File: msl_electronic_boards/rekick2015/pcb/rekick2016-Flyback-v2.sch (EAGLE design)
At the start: 201 parts, among them IC1 74LVC1G02GW, IC2 4043D, IC3 LM1117, IC4 LM1458D, P1 39-30-06_S, P2 39-30-08_S, Q1 16MHz, Q2 IKW 25N120, Q3 PSMN7R8-120PS, Q5 IPD90P04P4L, Q6 IRF840, T1 BC859, T2 BC849, T3 BC849, T4 BC849, T5 IRLML6344TRPBF, T6 BC859, U1 TXB0108PWR, U3 LM2675, U4 LM2675, U5 ADUM4190BRIZ, U6 ADUM4190BRIZ, X1 79109-12, X2 79109-04

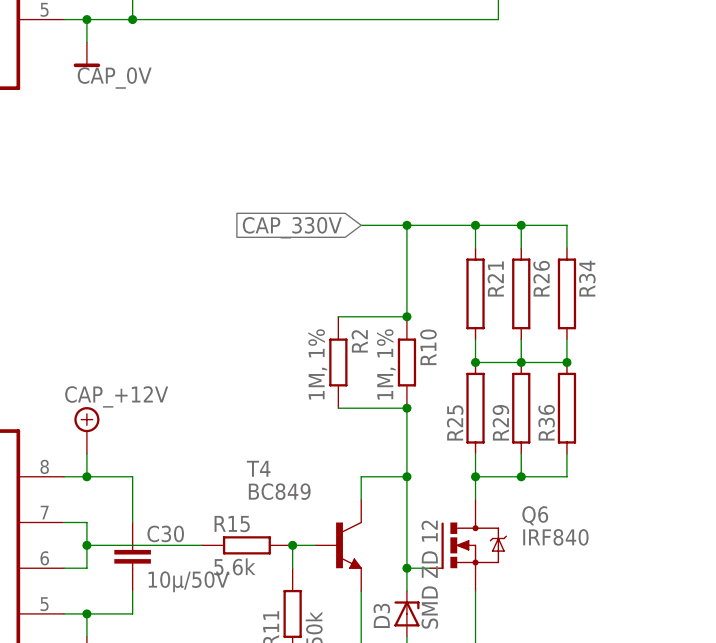
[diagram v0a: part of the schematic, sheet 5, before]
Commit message: rekick board  and  powerswitch board changes
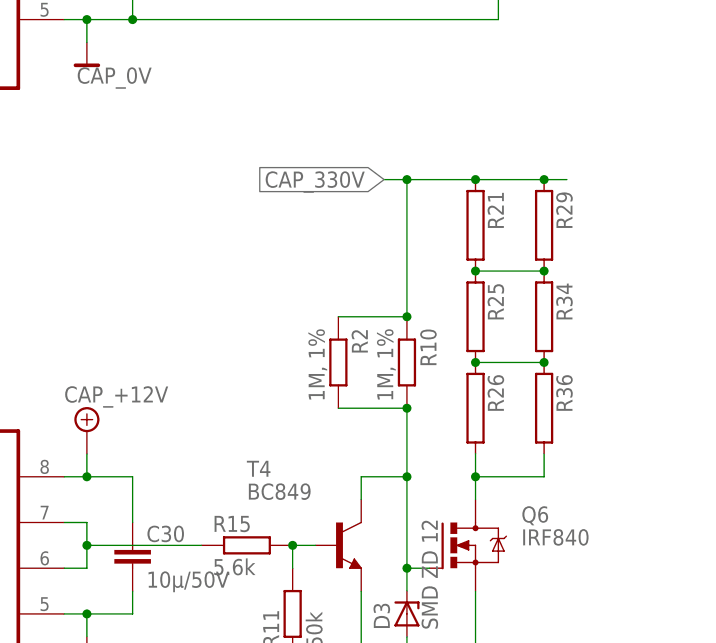
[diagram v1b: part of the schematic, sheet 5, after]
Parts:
- R21, R25, R26, R29, R34, R36: device resistor-power:RKH208-8R -> resistor-power:RKH214-8R
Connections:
- new net N$8: R25.2, R26.1, R34.2, R36.1
- net CAP_330V: now also R29.1; no longer R26.1, R34.1
- net N$13: now also R25.1, R34.1; no longer R25.2, R26.2, R34.2, R36.2
- net N$51: now also R26.2, R36.2; no longer R25.1, R29.1, R36.1
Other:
- moved on the sheet: R21, R25, R26, R29, R34, R36
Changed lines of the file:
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@@
 <part name="SUPPLY20" library="supply2" deviceset="0V" device="" value="CAP_0V"/>
 <part name="GND29" library="supply1" deviceset="GND" device=""/>
-<part name="R21" library="resistor-power" deviceset="R" device="KH208-8R"/>
-<part name="R25" library="resistor-power" deviceset="R" device="KH208-8R"/>
-<part name="R26" library="resistor-power" deviceset="R" device="KH208-8R"/>
-<part name="R29" library="resistor-power" deviceset="R" device="KH208-8R"/>
+<part name="R21" library="resistor-power" deviceset="R" device="KH214-8R"/>
+<part name="R25" library="resistor-power" deviceset="R" device="KH214-8R"/>
+<part name="R26" library="resistor-power" deviceset="R" device="KH214-8R"/>
+<part name="R29" library="resistor-power" deviceset="R" device="KH214-8R"/>
 <part name="FRAME8" library="frames" deviceset="A4L-LOC" device=""/>
 <part name="GND30" library="supply1" deviceset="GND" device=""/>
@@
 <part name="SUPPLY23" library="supply2" deviceset="GND1" device=""/>
 <part name="GND41" library="supply1" deviceset="GND" device=""/>
-<part name="R34" library="resistor-power" deviceset="R" device="KH208-8R"/>
-<part name="R36" library="resistor-power" deviceset="R" device="KH208-8R"/>
+<part name="R34" library="resistor-power" deviceset="R" device="KH214-8R"/>
+<part name="R36" library="resistor-power" deviceset="R" device="KH214-8R"/>
 <part name="X1" library="con-molex-milli-grid" deviceset="79109-12" device=""/>
 <part name="C43" library="rcl" deviceset="C-EU" device="C1206" value="10µ/50V"/>
@@
 <instance part="R11" gate="G$1" x="119.38" y="66.04" rot="R90"/>
 <instance part="R2" gate="G$1" x="124.46" y="93.98" rot="R270"/>
-<instance part="R21" gate="G$1" x="139.7" y="101.6" rot="R270"/>
-<instance part="R25" gate="G$1" x="139.7" y="88.9" rot="R90"/>
-<instance part="R26" gate="G$1" x="144.78" y="101.6" rot="R270"/>
-<instance part="R29" gate="G$1" x="144.78" y="88.9" rot="R90"/>
-<instance part="R34" gate="G$1" x="149.86" y="101.6" rot="R270"/>
-<instance part="R36" gate="G$1" x="149.86" y="88.9" rot="R90"/>
+<instance part="R21" gate="G$1" x="139.7" y="109.22" rot="R270"/>
+<instance part="R25" gate="G$1" x="139.7" y="99.06" rot="R270"/>
+<instance part="R26" gate="G$1" x="139.7" y="88.9" rot="R270"/>
+<instance part="R29" gate="G$1" x="147.32" y="109.22" rot="R270"/>
+<instance part="R34" gate="G$1" x="147.32" y="99.06" rot="R270"/>
+<instance part="R36" gate="G$1" x="147.32" y="88.9" rot="R270"/>
 </instances>
 <busses>
@@
 </segment>
 <segment>
-<label x="127" y="109.22" size="1.778" layer="95" rot="R180" xref="yes"/>
-<wire x1="127" y1="109.22" x2="132.08" y2="109.22" width="0.1524" layer="91"/>
+<label x="129.54" y="114.3" size="1.778" layer="95" rot="R180" xref="yes"/>
+<wire x1="129.54" y1="114.3" x2="132.08" y2="114.3" width="0.1524" layer="91"/>
 <pinref part="R10" gate="G$1" pin="1"/>
-<wire x1="132.08" y1="109.22" x2="139.7" y2="109.22" width="0.1524" layer="91"/>
-<wire x1="139.7" y1="109.22" x2="144.78" y2="109.22" width="0.1524" layer="91"/>
-<wire x1="144.78" y1="109.22" x2="149.86" y2="109.22" width="0.1524" layer="91"/>
-<wire x1="132.08" y1="99.06" x2="132.08" y2="109.22" width="0.1524" layer="91"/>
-<junction x="132.08" y="109.22"/>
+<wire x1="132.08" y1="114.3" x2="139.7" y2="114.3" width="0.1524" layer="91"/>
+<wire x1="139.7" y1="114.3" x2="147.32" y2="114.3" width="0.1524" layer="91"/>
+<wire x1="147.32" y1="114.3" x2="149.86" y2="114.3" width="0.1524" layer="91"/>
+<wire x1="132.08" y1="99.06" x2="132.08" y2="114.3" width="0.1524" layer="91"/>
+<junction x="132.08" y="114.3"/>
 <pinref part="R2" gate="G$1" pin="1"/>
 <wire x1="124.46" y1="99.06" x2="132.08" y2="99.06" width="0.1524" layer="91"/>
 <junction x="132.08" y="99.06"/>
 <pinref part="R21" gate="G$1" pin="1"/>
-<wire x1="139.7" y1="106.68" x2="139.7" y2="109.22" width="0.1524" layer="91"/>
-<junction x="139.7" y="109.22"/>
-<pinref part="R26" gate="G$1" pin="1"/>
-<wire x1="144.78" y1="106.68" x2="144.78" y2="109.22" width="0.1524" layer="91"/>
-<junction x="144.78" y="109.22"/>
-<pinref part="R34" gate="G$1" pin="1"/>
-<wire x1="149.86" y1="106.68" x2="149.86" y2="109.22" width="0.1524" layer="91"/>
+<junction x="139.7" y="114.3"/>
+<pinref part="R29" gate="G$1" pin="1"/>
+<junction x="147.32" y="114.3"/>
 </segment>
 </net>
@@
 <segment>
 <pinref part="Q6" gate="G$1" pin="D"/>
+<wire x1="139.7" y1="83.82" x2="139.7" y2="81.28" width="0.1524" layer="91"/>
+<pinref part="R26" gate="G$1" pin="2"/>
+<pinref part="R36" gate="G$1" pin="2"/>
+<wire x1="139.7" y1="81.28" x2="139.7" y2="78.74" width="0.1524" layer="91"/>
+<wire x1="139.7" y1="81.28" x2="147.32" y2="81.28" width="0.1524" layer="91"/>
+<wire x1="147.32" y1="81.28" x2="147.32" y2="83.82" width="0.1524" layer="91"/>
+<junction x="139.7" y="81.28"/>
+</segment>
+</net>
+<net name="N$8" class="0">
+<segment>
+<pinref part="R26" gate="G$1" pin="1"/>
+<pinref part="R25" gate="G$1" pin="2"/>
+<pinref part="R34" gate="G$1" pin="2"/>
+<pinref part="R36" gate="G$1" pin="1"/>
+<wire x1="139.7" y1="93.98" x2="147.32" y2="93.98" width="0.1524" layer="91"/>
+<junction x="139.7" y="93.98"/>
+<junction x="147.32" y="93.98"/>
+</segment>
+</net>
+<net name="N$13" class="0">
+<segment>
 <pinref part="R25" gate="G$1" pin="1"/>
-<wire x1="139.7" y1="83.82" x2="139.7" y2="81.28" width="0.1524" layer="91"/>
-<pinref part="R29" gate="G$1" pin="1"/>
-<wire x1="139.7" y1="81.28" x2="139.7" y2="78.74" width="0.1524" layer="91"/>
-<wire x1="144.78" y1="83.82" x2="144.78" y2="81.28" width="0.1524" layer="91"/>
-<wire x1="144.78" y1="81.28" x2="139.7" y2="81.28" width="0.1524" layer="91"/>
-<junction x="139.7" y="81.28"/>
-<pinref part="R36" gate="G$1" pin="1"/>
-<wire x1="149.86" y1="83.82" x2="149.86" y2="81.28" width="0.1524" layer="91"/>
-<wire x1="149.86" y1="81.28" x2="144.78" y2="81.28" width="0.1524" layer="91"/>
-<junction x="144.78" y="81.28"/>
-</segment>
-</net>
-<net name="N$13" class="0">
-<segment>
-<pinref part="R25" gate="G$1" pin="2"/>
 <pinref part="R21" gate="G$1" pin="2"/>
-<wire x1="139.7" y1="96.52" x2="139.7" y2="93.98" width="0.1524" layer="91"/>
 <pinref part="R29" gate="G$1" pin="2"/>
-<pinref part="R26" gate="G$1" pin="2"/>
-<wire x1="144.78" y1="96.52" x2="144.78" y2="93.98" width="0.1524" layer="91"/>
-<wire x1="139.7" y1="93.98" x2="144.78" y2="93.98" width="0.1524" layer="91"/>
-<junction x="139.7" y="93.98"/>
-<junction x="144.78" y="93.98"/>
-<pinref part="R36" gate="G$1" pin="2"/>
-<pinref part="R34" gate="G$1" pin="2"/>
-<wire x1="149.86" y1="96.52" x2="149.86" y2="93.98" width="0.1524" layer="91"/>
-<wire x1="144.78" y1="93.98" x2="149.86" y2="93.98" width="0.1524" layer="91"/>
-<junction x="149.86" y="93.98"/>
-</segment>
-</net>
+<pinref part="R34" gate="G$1" pin="1"/>
+<wire x1="139.7" y1="104.14" x2="147.32" y2="104.14" width="0.1524" layer="91"/>
+<junction x="139.7" y="104.14"/>
+<junction x="147.32" y="104.14"/>
+</segment>
+</net>
